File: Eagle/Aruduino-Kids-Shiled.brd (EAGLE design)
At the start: 86.4 x 52.8 mm, 17 parts

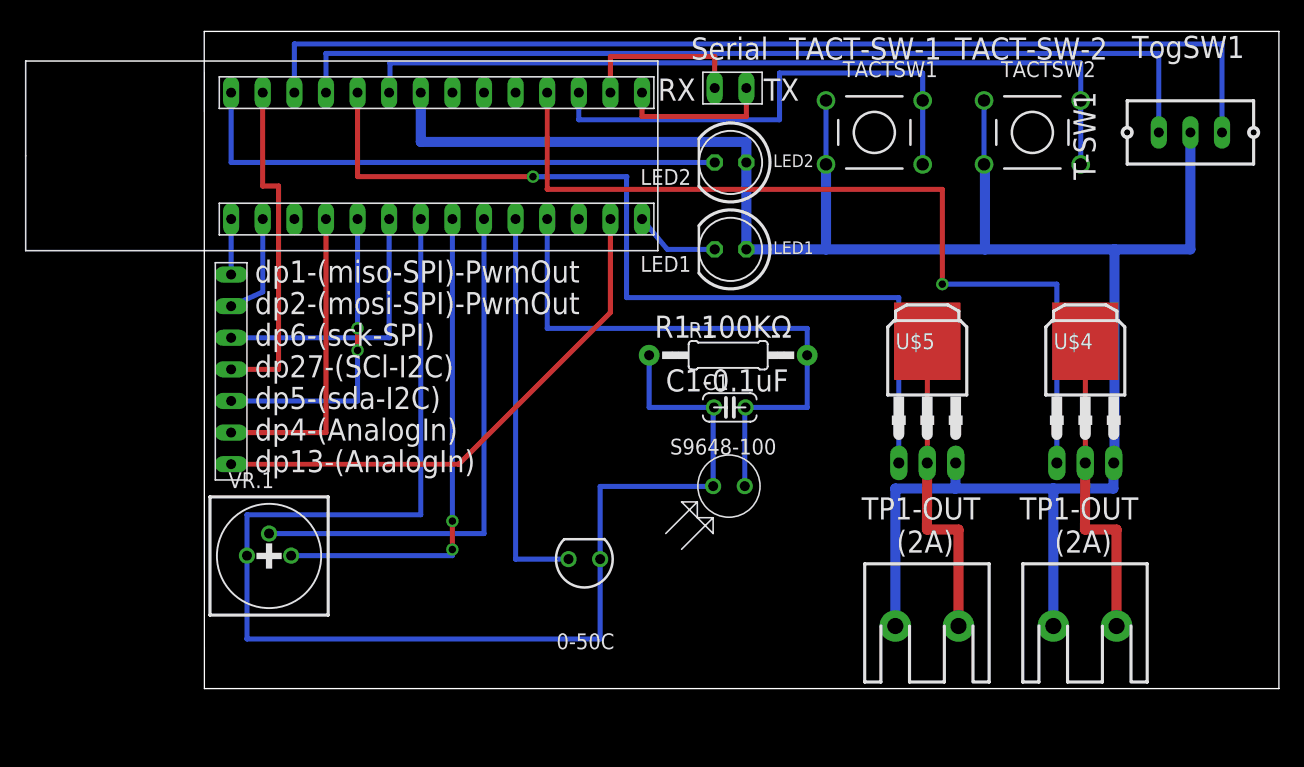
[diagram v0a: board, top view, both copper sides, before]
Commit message: Semi_Final
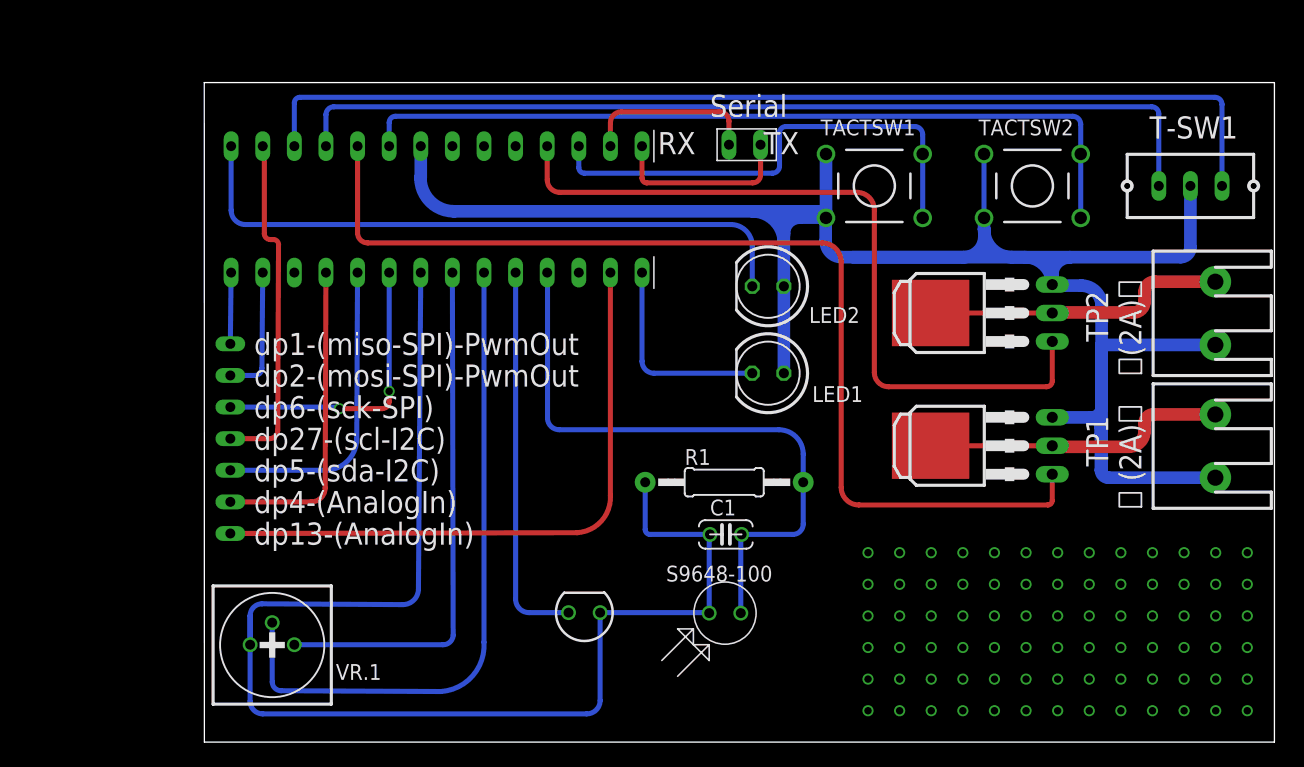
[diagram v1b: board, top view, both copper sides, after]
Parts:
- moved TB2 27.3 mm to (81.3, 23.8), turned to 0 degrees
- moved TB1 27.2 mm to (81.3, 34.5), turned to 0 degrees
- moved U$4 11.3 mm to (60.3, 34.5), turned to 90 degrees
- moved LED1 10.4 mm to (45.3, 29.7)
- moved LED2 10.4 mm to (45.3, 36.6)
- moved U$2 10.2 mm to (41.8, 10.4)
- moved R1 10.2 mm to (41.8, 20.9)
- moved C1 10.2 mm to (41.9, 16.7)
- moved VR.1 7.16 mm to (5.46, 7.82)
- moved U$5 6.85 mm to (60.3, 23.8), turned to 90 degrees
- moved U$3 5.57 mm to (2.10, 24.4)
- moved U$6 4.70 mm to (43.4, 48.0)
- moved T-SW1 4.30 mm to (79.2, 44.7)
- moved TACTSW1 4.30 mm to (53.8, 44.7)
- moved TACTSW2 4.30 mm to (66.5, 44.7)
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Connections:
- net N$1 renamed GND
- net N$19 renamed P18
- net N$2 renamed P14
- net N$20 renamed P24
- net N$3 renamed P28
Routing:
- net P24: track 73.3 -> 84.8 mm, vias 1 -> 0
- net GND: track 168.8 -> 180.0 mm
- net N$8: track 42.5 -> 53.6 mm
- net P18: track 70.7 -> 61.2 mm, vias 1 -> 0
- net P14: track 6.98 -> 16.4 mm
- net P28: track 44.5 -> 51.5 mm
- net N$25: track 43.0 -> 49.8 mm
- net N$6: track 113.2 -> 107.0 mm
- net N$5: track 47.4 -> 50.8 mm
- net N$27: track 12.6 -> 14.9 mm
- net N$99: track 0.00 -> 2.31 mm
- net N$7: track 40.0 -> 42.2 mm, vias 2 -> 0
- net N$14: track 8.64 -> 10.5 mm
- net N$9: track 40.9 -> 39.6 mm
- net N$10: track 4.46 -> 5.73 mm
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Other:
- board size 86.4 x 52.8 mm -> 86 x 53 mm
- board text added: "TP1 ー (2A)＋"
- board text added: "TP2 ー(2A)＋"
- board text added: "Tr1"
- board text added: "Tr2"
- board text added: "dp27-(scl-I2C)"
- board text removed: "C1-0.1uF"
- board text removed: "LED1"
- board text removed: "LED2"
- board text removed: "R1-100KΩ"
- board text removed: "TACT-SW-1"
- board text removed: "TACT-SW-2"
- board text removed: "TP1-OUT (2A)"
- board text removed: "TogSW1"
- board text removed: "dp27-(SCl-I2C)"
